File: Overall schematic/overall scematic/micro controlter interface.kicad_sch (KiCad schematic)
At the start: 5 parts, among them J10 Conn_01x09_Pin, J8 DB25_Receptacle, J9 DB25_Receptacle, U3 STLINK_UCT, U4 AT24CS01-STUM

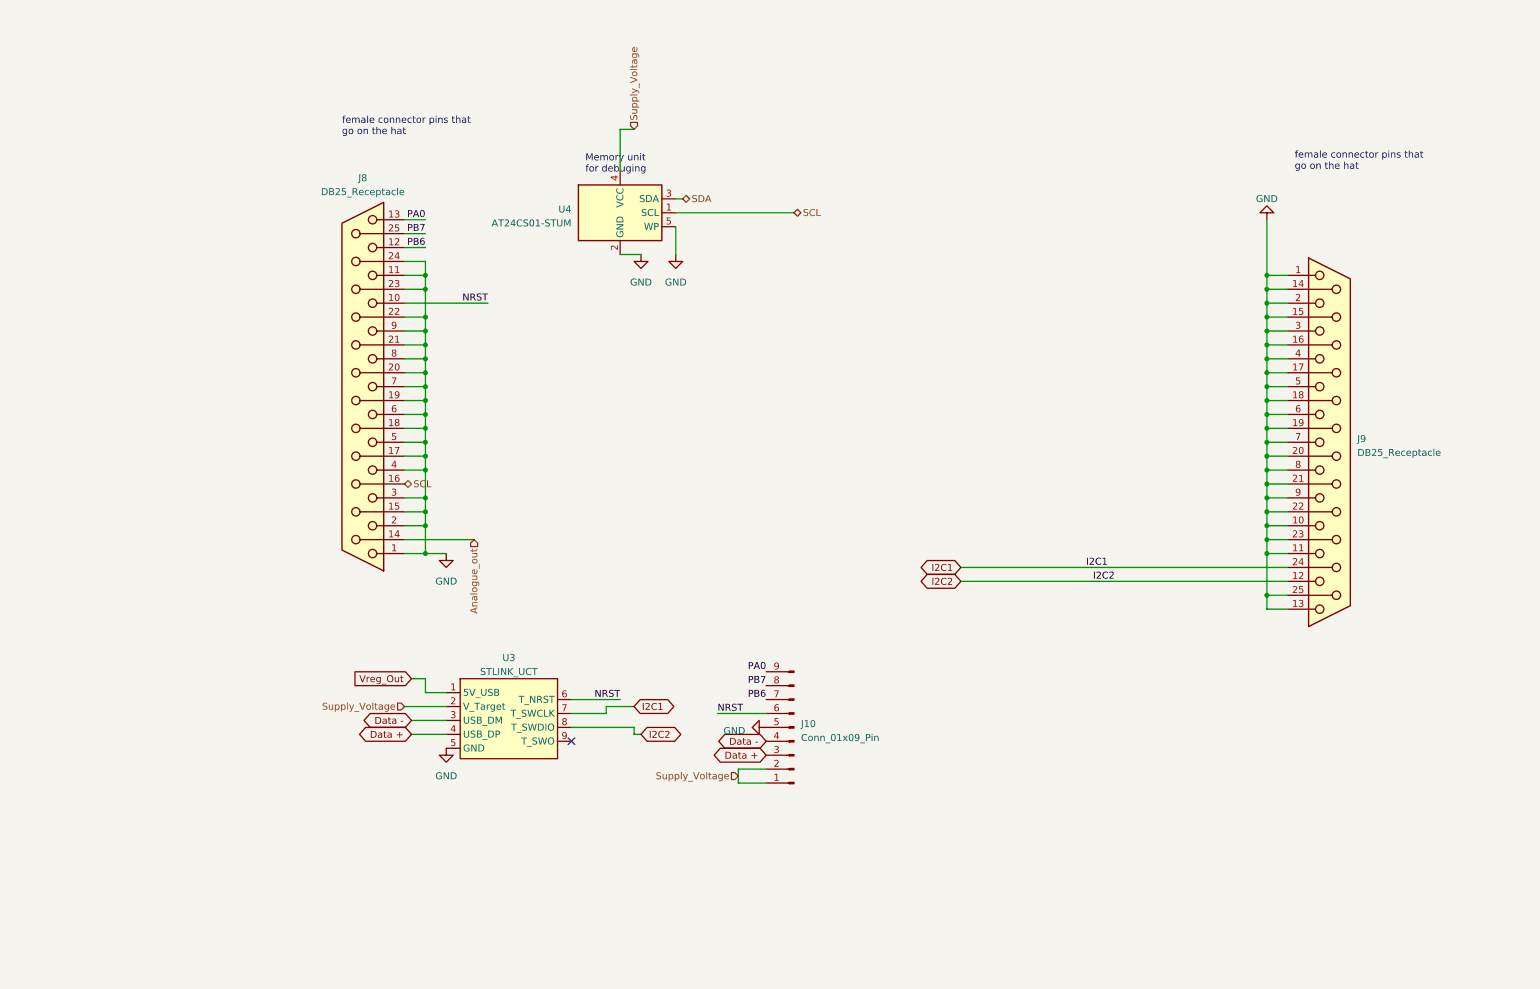
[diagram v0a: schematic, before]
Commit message: hail mary
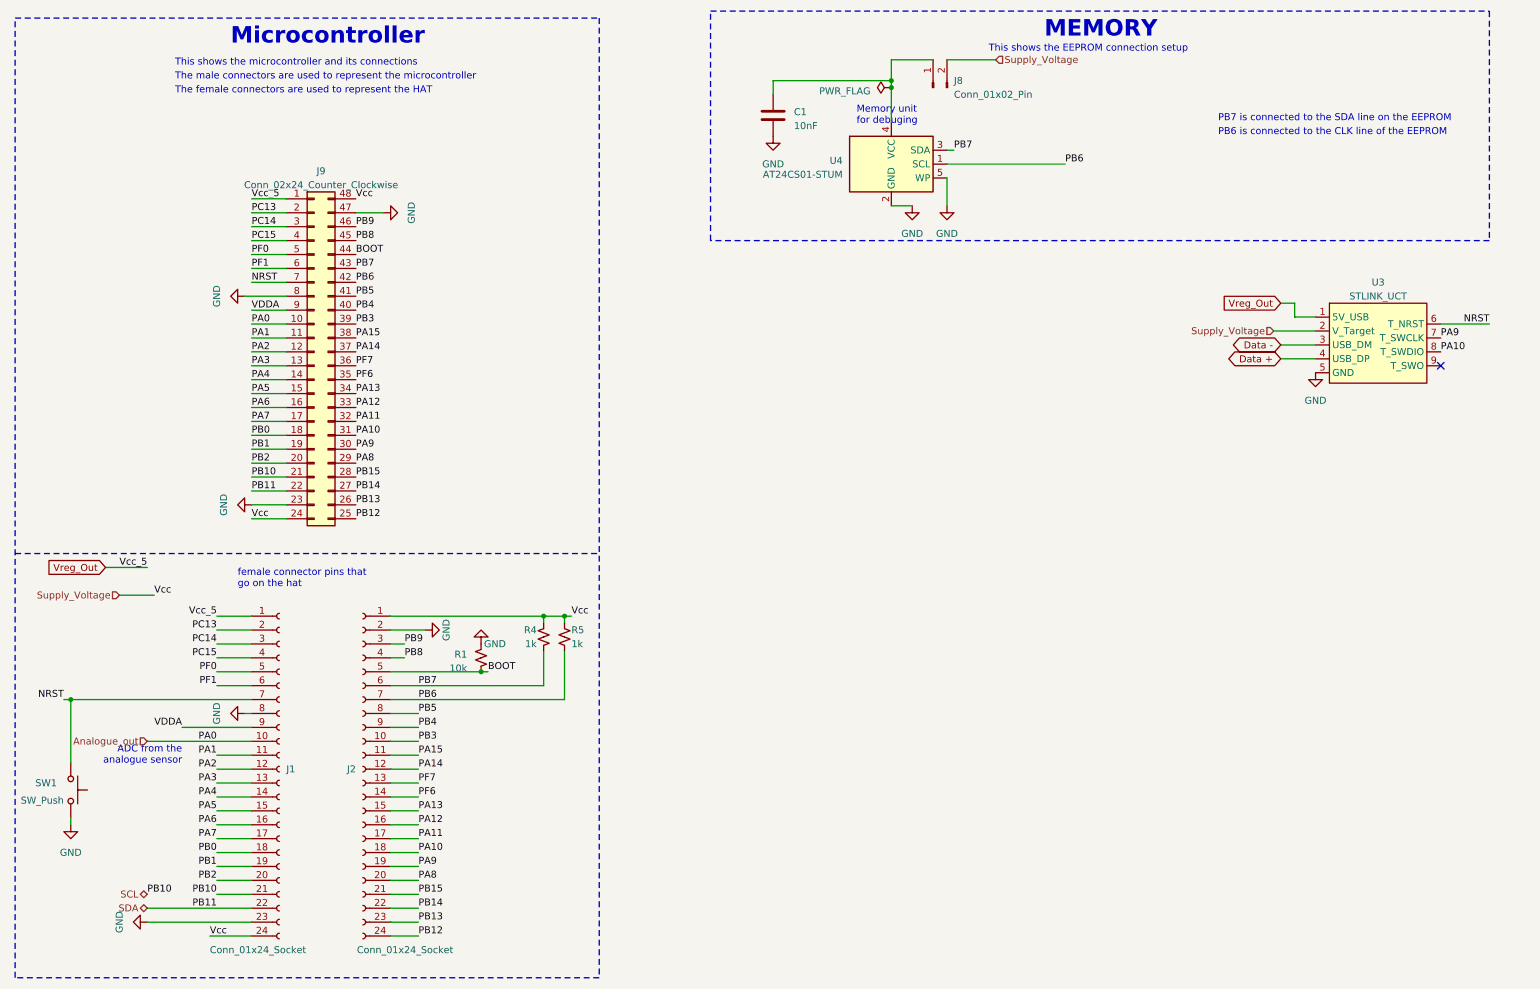
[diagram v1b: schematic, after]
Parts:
- removed J10: Conn_01x09_Pin, Connector_PinHeader_2.54mm:PinHeader_1x03_P2.54mm_Vertical, symbol Connector:Conn_01x09_Pin
- removed J8, J9: DB25_Receptacle, SSQ-120-03-G-D:SAMTEC_SSQ-120-03-G-D, symbol Custom spi connector:DB25_Receptacle
- added C1: 10nF, Capacitor_SMD:C_1206_3216Metric, symbol Device:C
- added J1, J2: Conn_01x24_Socket, BAT60JFILM:SAMTEC_SSQ-120-03-G-D, symbol Connector:Conn_01x24_Socket
- added J8: Conn_01x02_Pin, Connector_PinHeader_2.54mm:PinHeader_1x02_P2.54mm_Vertical, symbol Connector:Conn_01x02_Pin
- added J9: Conn_02x24_Counter_Clockwise, BAT60JFILM:STM32F051C6T6, symbol Connector_Generic:Conn_02x24_Counter_Clockwise
- added R1: 10k, Resistor_SMD:R_0805_2012Metric, symbol Device:R_Small_US
- added R4, R5: 1k, Resistor_SMD:R_0603_1608Metric, symbol Device:R_Small_US
- added SW1: SW_Push, Button_Switch_THT:SW_PUSH_6mm, symbol Switch:SW_Push
- U3: footprint Module:ST_Morpho_Connector_144_STLink -> BAT60JFILM:STLINK_UCT
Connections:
- net Analogue_out: now also J1.10 (Pin_10), J9.10 (Pin_10)
- net GND: now also C1.2, J1.23 (Pin_23), J1.8 (Pin_8), J2.2 (Pin_2), J9.23 (Pin_23), J9.47 (Pin_47), J9.8 (Pin_8), R1.1, SW1.1
- net NRST: now also J1.7 (Pin_7), J9.7 (Pin_7), SW1.2
- net PB6: now also U4.1 (SCL), J2.7 (Pin_7), J9.42 (Pin_42), R5.2
- net PB7: now also U4.3 (SDA), J2.6 (Pin_6), J9.43 (Pin_43), R4.2
- net SCL: now also J1.21 (Pin_21), J9.21 (Pin_21); no longer U4.1 (SCL)
- net SDA: now also J1.22 (Pin_22), J9.22 (Pin_22); no longer U4.3 (SDA)
- net Supply_Voltage: now also J1.24 (Pin_24), J2.1 (Pin_1), J8.2 (Pin_2), J9.24 (Pin_24), J9.48 (Pin_48), R4.1, R5.1; no longer U4.4 (VCC)
- net Vreg_Out: now also J1.1 (Pin_1), J9.1 (Pin_1)
- net I2C1 renamed PA9
- net PA9: now also J2.19 (Pin_19), J9.30 (Pin_30)
- net I2C2 renamed PA10
- net PA10: now also J2.18 (Pin_18), J9.31 (Pin_31)
- new net: C1.1, J8.1 (Pin_1), U4.4 (VCC)
- new net BOOT: J2.5 (Pin_5), J9.44 (Pin_44), R1.2
- new net PA1: J1.11 (Pin_11), J9.11 (Pin_11)
- new net PA11: J2.17 (Pin_17), J9.32 (Pin_32)
- new net PA12: J2.16 (Pin_16), J9.33 (Pin_33)
- new net PA13: J2.15 (Pin_15), J9.34 (Pin_34)
- new net PA14: J2.12 (Pin_12), J9.37 (Pin_37)
- new net PA15: J2.11 (Pin_11), J9.38 (Pin_38)
- new net PA2: J1.12 (Pin_12), J9.12 (Pin_12)
- new net PA3: J1.13 (Pin_13), J9.13 (Pin_13)
- new net PA4: J1.14 (Pin_14), J9.14 (Pin_14)
- new net PA5: J1.15 (Pin_15), J9.15 (Pin_15)
- new net PA6: J1.16 (Pin_16), J9.16 (Pin_16)
- new net PA7: J1.17 (Pin_17), J9.17 (Pin_17)
- new net PA8: J2.20 (Pin_20), J9.29 (Pin_29)
- new net PB0: J1.18 (Pin_18), J9.18 (Pin_18)
- new net PB1: J1.19 (Pin_19), J9.19 (Pin_19)
- new net PB12: J2.24 (Pin_24), J9.25 (Pin_25)
- new net PB13: J2.23 (Pin_23), J9.26 (Pin_26)
- new net PB14: J2.22 (Pin_22), J9.27 (Pin_27)
- new net PB15: J2.21 (Pin_21), J9.28 (Pin_28)
- new net PB2: J1.20 (Pin_20), J9.20 (Pin_20)
- new net PB3: J2.10 (Pin_10), J9.39 (Pin_39)
- new net PB4: J2.9 (Pin_9), J9.40 (Pin_40)
- new net PB5: J2.8 (Pin_8), J9.41 (Pin_41)
- new net PB8: J2.4 (Pin_4), J9.45 (Pin_45)
- new net PB9: J2.3 (Pin_3), J9.46 (Pin_46)
- new net PC13: J1.2 (Pin_2), J9.2 (Pin_2)
- new net PC14: J1.3 (Pin_3), J9.3 (Pin_3)
- new net PC15: J1.4 (Pin_4), J9.4 (Pin_4)
- new net PF0: J1.5 (Pin_5), J9.5 (Pin_5)
- new net PF1: J1.6 (Pin_6), J9.6 (Pin_6)
- new net PF6: J2.14 (Pin_14), J9.35 (Pin_35)
- new net PF7: J2.13 (Pin_13), J9.36 (Pin_36)
- new net VDDA: J1.9 (Pin_9), J9.9 (Pin_9)
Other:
- note added: "ADC from the analogue sensor"
- note added: "MEMORY"
- note added: "Microcontroller"
- note added: "PB6 is connected to the CLK line of the EEPROM"
- note added: "PB7 is connected to the SDA line on the EEPROM"
- note added: "The female connectors are used to represent the HAT"
- note added: "The male connectors are used to represent the microcontroller"
- note added: "This shows the EEPROM connection setup"
- note added: "This shows the microcontroller and its connections"
- moved on the sheet: U3, U4

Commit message: hail marry
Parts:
- J1, J2: footprint BAT60JFILM:SAMTEC_SSQ-120-03-G-D -> (none)
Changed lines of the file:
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@@
       (effects (font (size 1.27 1.27)) (justify left))
     )
-    (property "Footprint" "BAT60JFILM:SAMTEC_SSQ-120-03-G-D" (at 62.23 151.13 0)
+    (property "Footprint" "" (at 62.23 151.13 0)
       (effects (font (size 1.27 1.27)) hide)
     )
@@
       (effects (font (size 1.27 1.27)) (justify left))
     )
-    (property "Footprint" "BAT60JFILM:SAMTEC_SSQ-120-03-G-D" (at 77.47 151.13 0)
-      (effects (font (size 1.27 1.27)) hide)
-    )
+    (property "Footprint" "" (at 77.47 151.13 0)
+      (effects (font (size 1.27 1.27)) hide)
+    )
